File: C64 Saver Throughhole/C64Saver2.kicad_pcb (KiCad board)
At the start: 2 copper layers, 43.9 x 28.8 mm, 24 parts, among them J1 Conn_01x04, J2 Conn_01x08, J4 Conn_01x08, J5 Conn_01x04, J6 Conn_01x04, Q1 BC547, Q2 IRFR5305, U1 TL431LP

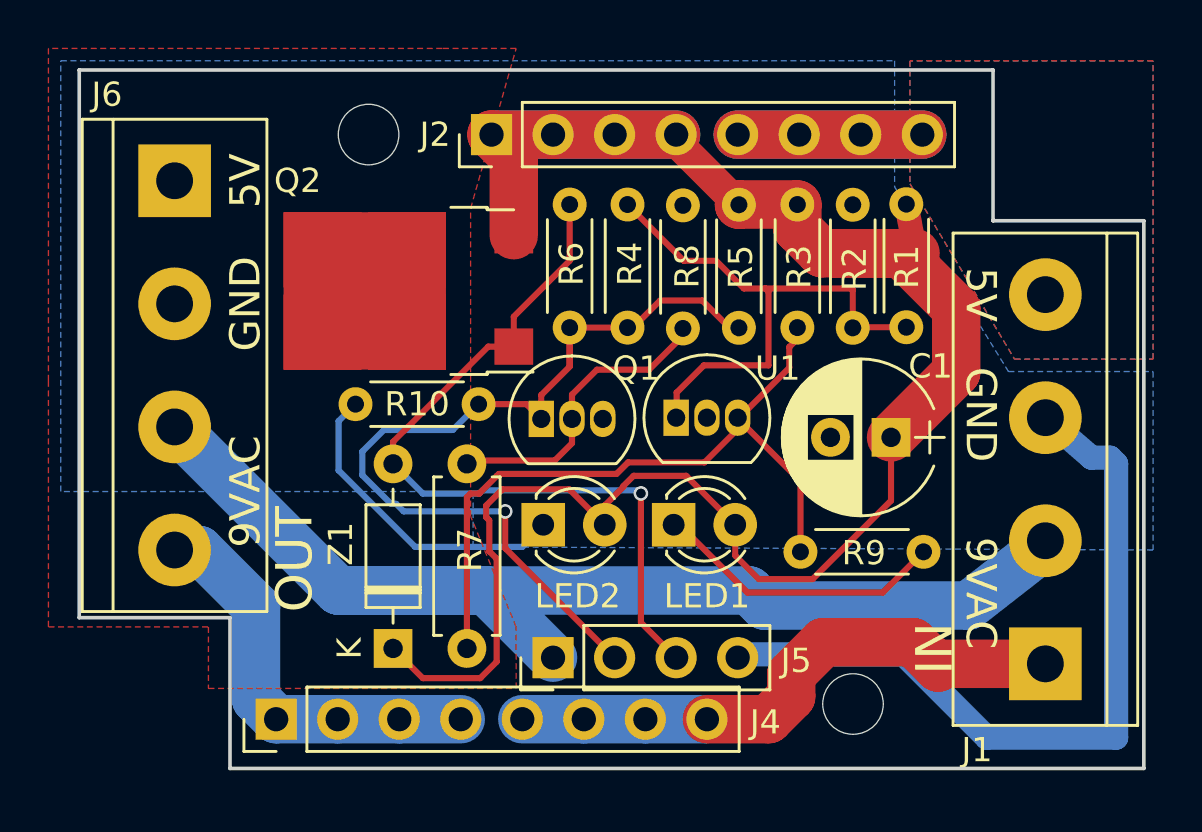
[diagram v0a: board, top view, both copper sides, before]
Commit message: 2.7 with iBom and gerbers
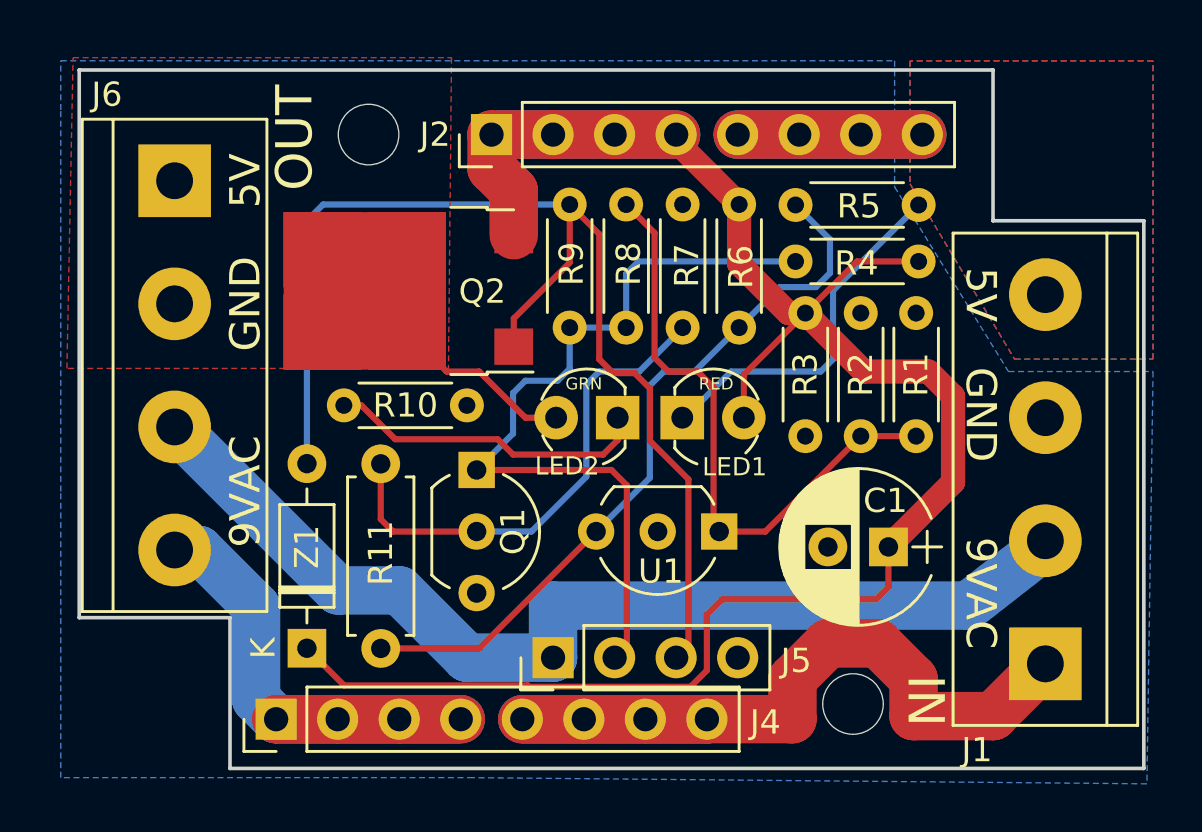
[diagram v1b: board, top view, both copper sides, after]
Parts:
- added R2: 330 1%, Resistor_THT:R_Axial_DIN0204_L3.6mm_D1.6mm_P5.08mm_Horizontal, F.Cu at (172.7, 93.7)
- LED1: footprint LED_THT:LED_D3.0mm -> LED_THT:LED_D3.0mm_Easy_1
- LED2: footprint LED_THT:LED_D3.0mm -> LED_THT:LED_D3.0mm_Easy_2
- Q1, U1: footprint Package_TO_SOT_THT:TO-92_Inline -> Package_TO_SOT_THT:TO-92_Inline_Wide
- Q2: value IRFR5305 -> IPD068P03L3G
- R10: value 1k -> 330
- R3: renamed from R1; value 3k9 1% -> 3k3 1%
- moved R5 14.3 mm to (175.1, 89.3)
- moved R4 7.78 mm to (175.1, 91.6), turned to 180 degrees
- moved R3 6.13 mm to (170.4, 93.7)
- moved LED2 5.38 mm to (162.7, 98.0), turned to 180 degrees
- moved R1 5.18 mm to (175.0, 98.8)
- moved U1 5.02 mm to (166.9, 102.7), turned to 180 degrees
- moved C1 4.52 mm to (173.9, 103.4)
- moved LED1 4.43 mm to (165.4, 98.0)
- moved Z1 3.56 mm to (149.9, 107.6)
- moved R11 3.56 mm to (152.9, 107.6)
- moved Q1 3.40 mm to (156.9, 100.2), turned to -90 degrees
- moved R6 2.40 mm to (167.7, 89.2)
- moved R10 0.49 mm to (151.4, 97.5)
- moved R8 0.06 mm to (163.0, 89.2)
- renumbered R2 to R1, R7 to R11, R5 to R4, R9 to R5, R3 to R6, R8 to R7, R4 to R8, R6 to R9
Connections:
- LED2 pad 2: /VCC1- -> /5V_SAFE
- R10 pad 2: OVERVOLTAGE -> GND
- R3 pad 2: /SENSE -> unconnected-(R3-Pad2)
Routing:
- net GND: track 32.0 -> 0.19 mm
- net PGATE: track 32.6 -> 49.4 mm, vias 1 -> 0
- net /9VAC1: track 23.9 -> 34.5 mm
- net /NGATE: track 12.7 -> 20.7 mm
- net /9VAC1': track 16.9 -> 24.6 mm
- net /5V_SAFE: track 0.00 -> 7.61 mm
- net /9VAC2: track 50.2 -> 43.2 mm
- net OVERVOLTAGE: track 37.9 -> 33.8 mm, vias 1 -> 0
- net Net-(LED1-K): track 12.2 -> 15.1 mm
- net /SENSE: track 23.1 -> 25.6 mm
- net /VCC1-: track 84.0 -> 84.9 mm
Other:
- rule pad_to_mask_clearance: 0.2 -> 0
- board text added: "C64 Saver 2 THT version Rev 2.7 BWACK, Everlast 2023"
- board text added: "GRN"
- board text added: "RED"
- board text removed: "C64 Saver 2 THT version Rev 2.6 BWACK 2023"
